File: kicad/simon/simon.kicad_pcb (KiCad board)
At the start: 2 copper layers, 99.8 x 99.8 mm, 20 parts, among them J1 GPIO, J2 Power, U1 74LS06

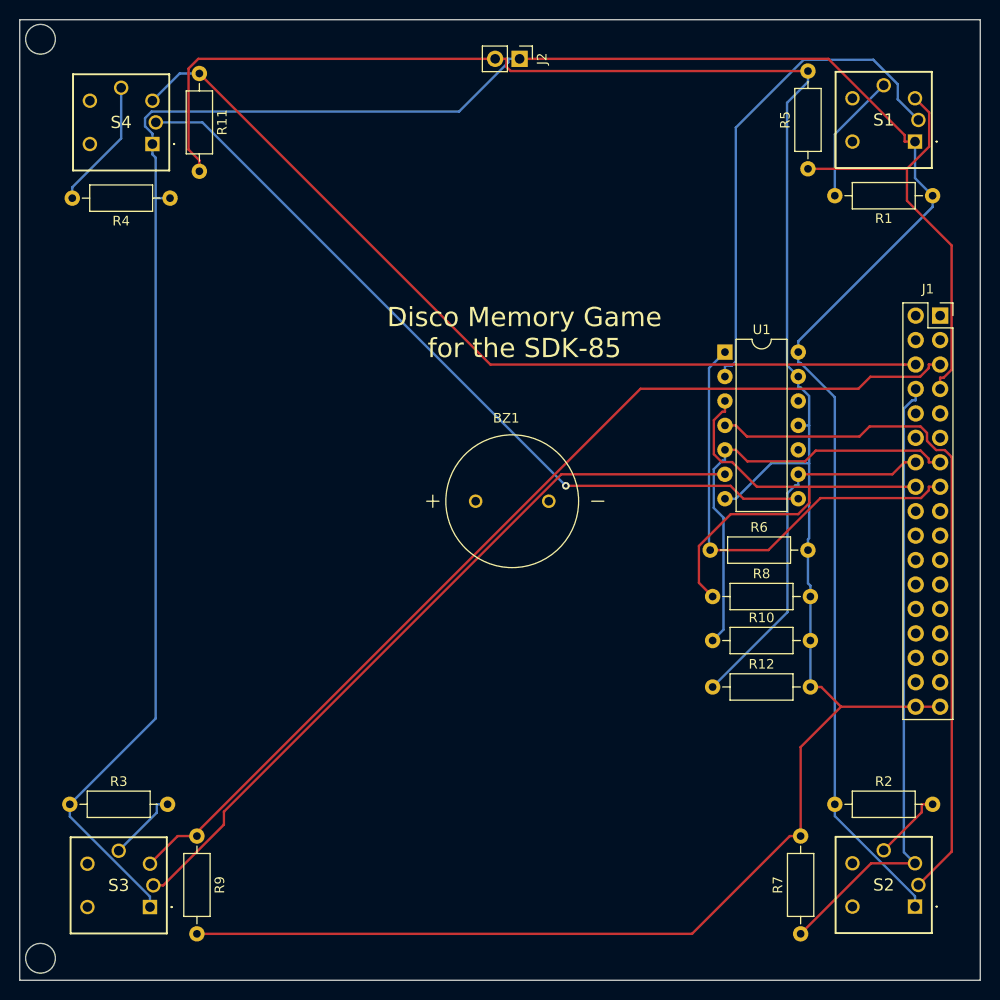
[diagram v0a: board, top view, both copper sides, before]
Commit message: Production version of Simon board.
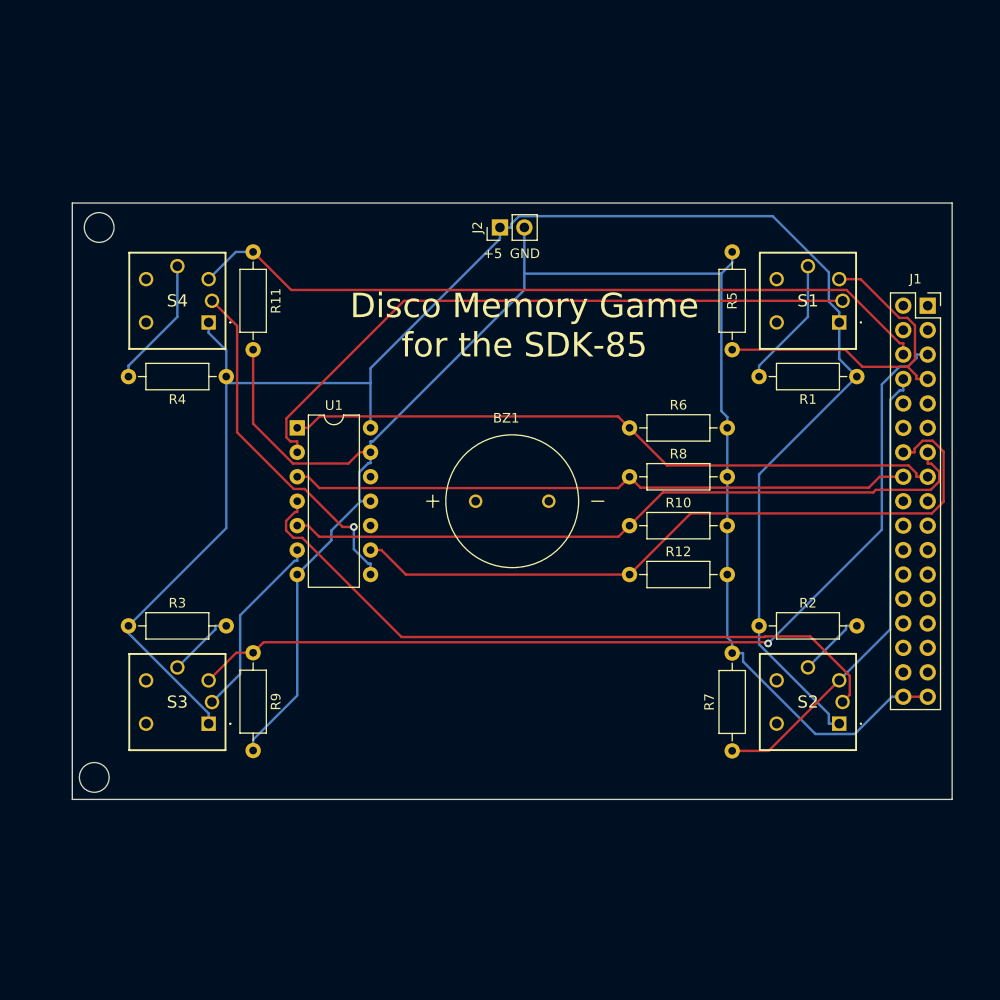
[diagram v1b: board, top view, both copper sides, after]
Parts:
- moved U1 45.1 mm to (156.5, 83.6)
- moved S2 20.6 mm to (212.8, 114.3)
- moved R5 20.4 mm to (201.7, 75.4)
- moved S1 20.4 mm to (212.8, 72.6)
- moved R1 20.4 mm to (214.6, 78.2)
- moved R7 20.3 mm to (201.7, 117.1)
- moved R2 20.1 mm to (204.5, 104.1)
- moved S3 20.0 mm to (147.3, 114.3)
- moved R9 19.9 mm to (151.9, 106.9)
- moved R3 19.5 mm to (138.9, 104.1)
- moved R4 19.4 mm to (149.1, 78.2)
- moved S4 19.4 mm to (147.3, 72.6)
- moved R11 19.4 mm to (151.9, 65.3)
- moved J2 17.6 mm to (177.5, 62.7), turned to 90 degrees
- moved R6 15.2 mm to (191.0, 83.6)
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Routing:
- net VCC: track 269.0 -> 185.2 mm
- net GND: track 251.0 -> 178.6 mm
- net Net-(S3-K): track 77.9 -> 19.6 mm
- net Net-(S4-K): track 83.0 -> 36.8 mm
- net LT3: track 38.7 -> 74.3 mm
- net LT2: track 45.4 -> 73.3 mm
- net LT0: track 48.2 -> 68.8 mm
- net SW1: track 65.4 -> 48.4 mm
- net LT1: track 49.4 -> 64.9 mm
- net Net-(S1-K): track 52.1 -> 67.3 mm
- net SW3: track 93.0 -> 78.5 mm
- net SW0: track 44.7 -> 36.3 mm
- net SW2: track 104.0 -> 97.9 mm, vias 0 -> 1
- net Net-(S2-K): track 72.2 -> 71.6 mm
- net Net-(S3-A): track 7.59 -> 7.08 mm
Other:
- board size 99.8 x 99.8 mm -> 91.4 x 62 mm
- board text added: "+5"
- board text added: "GND"
